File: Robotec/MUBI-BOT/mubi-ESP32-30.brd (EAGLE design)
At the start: 70.2 x 49.5 mm, 35 parts, among them IC1 L293D, IC2 7805T

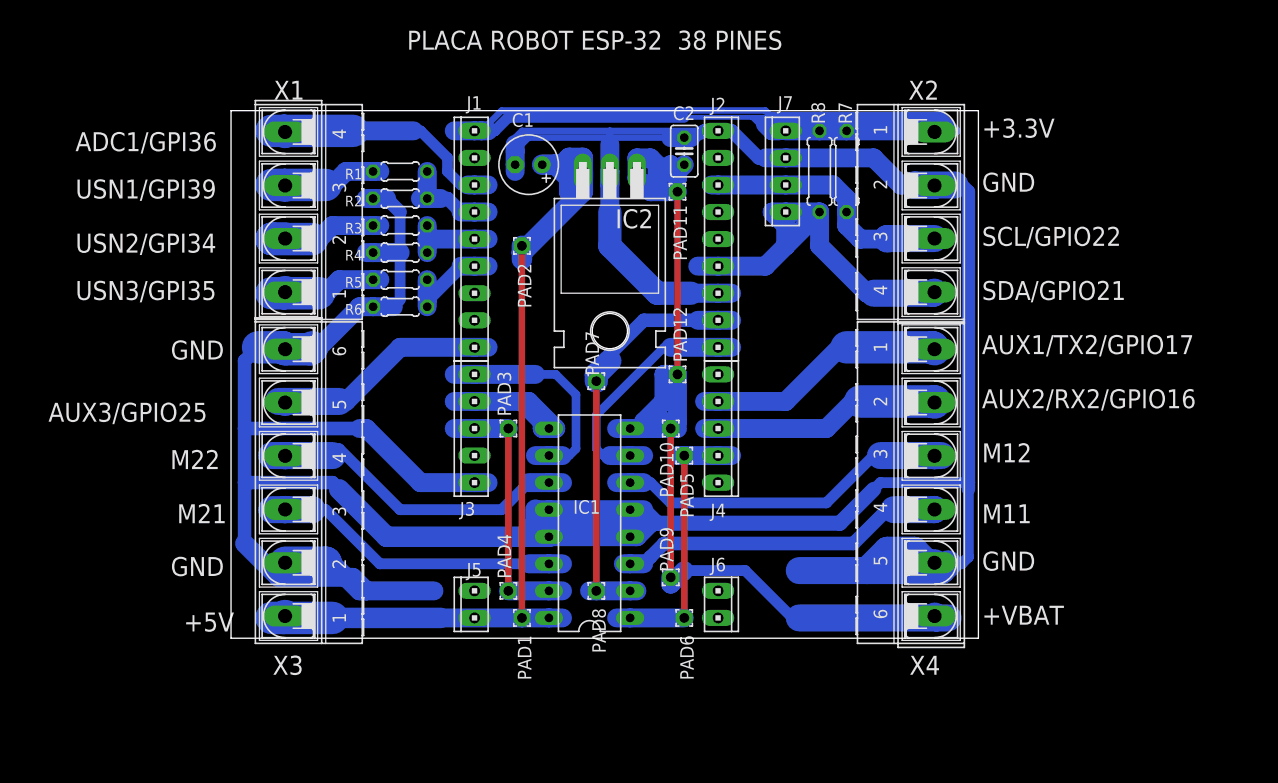
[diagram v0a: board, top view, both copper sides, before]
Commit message: update sch & brd
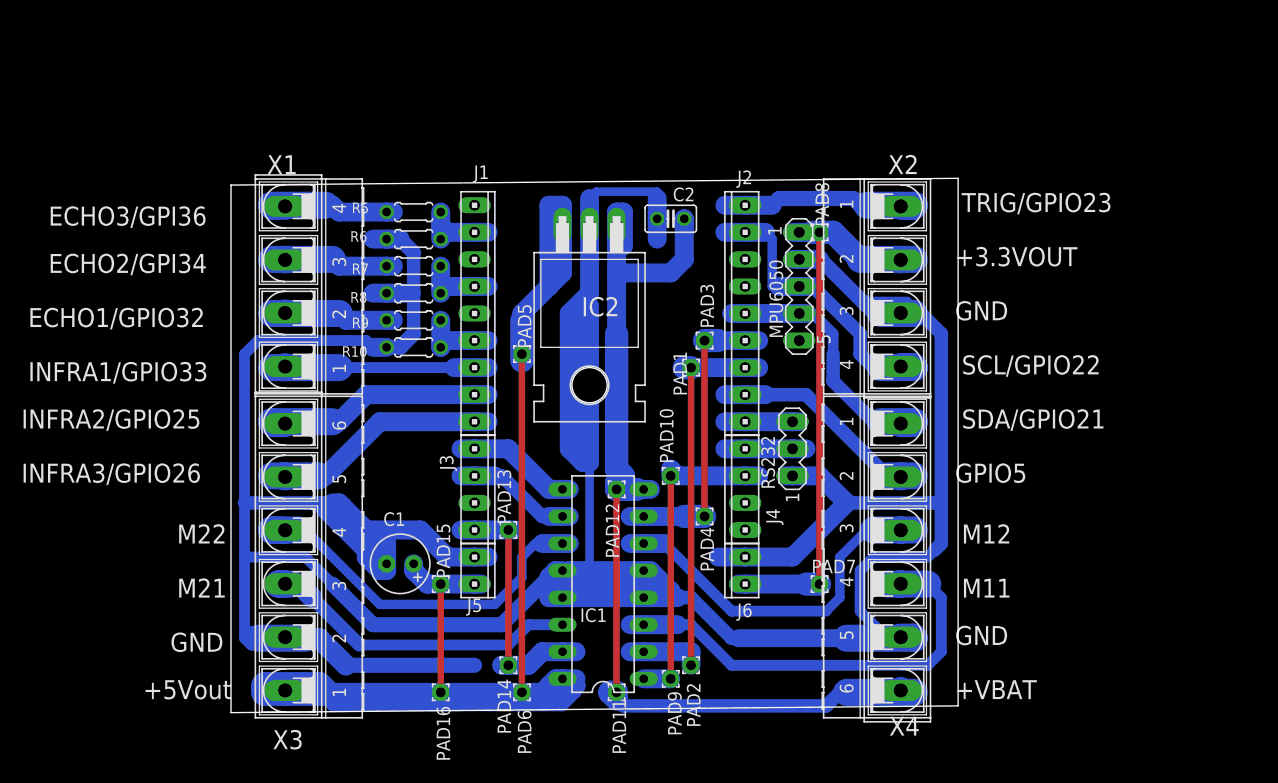
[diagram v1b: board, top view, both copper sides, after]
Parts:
- removed J7: (no value), con-amp:10X04MTA
- removed R1, R3: 5K6, resistor:0204/5
- removed R2, R4: 10K, resistor:0204/5
- added MPU6050: (no value), con-lstb:MA05-1
- added PAD13, PAD14, PAD15, PAD16: WIREPAD1,6/0,9, wirepad:1,6/0,9
- added R10: 10K, resistor:0204/5
- added R9: 5K6, resistor:0204/5
- added RS232: (no value), con-lstb:MA03-1
- C1: value 10uF/16V -> (none)
- C2: value 100nF -> (none)
- J3, J4: device con-amp:10X05MTA -> con-amp:10X04MTA
- R7: value 4K7 -> 5K6; device resistor:0207/7 -> resistor:0204/5
- R8: value 4K7 -> 10K; device resistor:0207/7 -> resistor:0204/5
- moved PAD11 47.3 mm to (36.2, 1.91)
- moved PAD2 42.5 mm to (43.2, 4.45)
- moved R7 41.6 mm to (17.1, 41.9), turned to 0 degrees
- moved R8 39.8 mm to (17.1, 39.4), turned to 180 degrees
- moved PAD8 39.6 mm to (55.2, 45.1)
- moved C1 39.4 mm to (15.9, 14.0)
- moved PAD1 28.4 mm to (43.2, 32.4)
- moved PAD7 28.3 mm to (55.2, 12.1)
- moved PAD3 20.2 mm to (44.5, 34.9)
- moved PAD4 19.7 mm to (44.5, 18.4)
- moved PAD5 18.0 mm to (27.3, 33.7)
- moved PAD6 16.8 mm to (27.3, 1.91)
- moved PAD12 12.2 mm to (36.2, 21.0), turned to 0 degrees
- moved PAD9 9.52 mm to (41.3, 3.17)
- moved X2 7.67 mm to (62.9, 40.0)
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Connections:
- removed net AUX1/TX2: J4.4, X4.1
- removed net AUX2/RX2: J4.3, X4.2
- removed net AUX3: J1.9, X3.5
- removed net N$1: R1.1, X1.3
- removed net N$2: R3.1, X1.2
- removed net N$4: J1.3, X1.4
- removed net USON1: J1.4, R1.2, R2.2
- removed net USON2: J1.5, R3.2, R4.2
- removed net USON3: J1.6, R5.2, R6.2
- new net GPI34: J1.6, R7.2, R8.1
- new net GPI36: J1.8, R5.2, R6.1
- new net GPIO23: J2.1, X2.1
- new net GPIO25: J1.2, X3.6
- new net GPIO26: J1.1, X3.5
- new net GPIO32: J1.4, R10.1, R9.2
- new net GPIO33: J1.3, X1.1
- new net GPIO5: J2.8, X4.2
- new net N$5: R7.1, X1.3
- new net N$8: R9.1, X1.2
- new net RX2: J4.1, RS232.2
- new net TX2: J2.9, RS232.3
- net +3.3V: now also J6.2, MPU6050.1, PAD7.1, PAD8.1, X2.2; no longer J1.1, J7.1, R7.2, R8.2, X2.1
- net +5V: now also J5.1, PAD15.1, PAD16.1, PAD5.1, PAD6.1; no longer J5.2, PAD1.1, PAD2.1
- net +VBAT: no longer PAD10.1, PAD9.1
- net CM11: now also J2.7, PAD1.1, PAD2.1; no longer J2.2, PAD7.1, PAD8.1
- net CM12: now also J2.6, PAD3.1, PAD4.1; no longer J2.1
- net CM21: now also J3.1, PAD13.1, PAD14.1; no longer J3.3, PAD3.1, PAD4.1
- net CM22: now also J3.3; no longer J3.1
- net ENAM1: now also PAD10.1, PAD9.1; no longer PAD5.1, PAD6.1
- net ENAM2: now also J3.4; no longer J3.2
- net GND: now also J5.2, J6.1, MPU6050.2, R10.2, R6.2, R8.2, RS232.1, X2.3; no longer J2.3, J2.9, J3.5, J7.2, R2.1, R4.1, R6.1, X2.2, X3.6
- net N$3: now also X1.4; no longer X1.1
- net SCL: now also J2.2, MPU6050.3, X2.4; no longer J2.7, J7.3, R7.1, X2.3
- net SDA: now also J2.5, MPU6050.4, X4.1; no longer J2.4, J7.4, R8.1, X2.4
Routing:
- net +5V: track 84.6 -> 167.8 mm
- net +3.3V: track 110.5 -> 53.2 mm
- net GND: track 358.7 -> 411.5 mm
- net AUX1/TX2: track 23.8 -> 0.00 mm
- net N$4: track 23.3 -> 0.00 mm
- net AUX2/RX2: track 22.7 -> 0.00 mm
- net GPIO25: track 0.00 -> 22.7 mm
- net GPIO26: track 0.00 -> 22.6 mm
- net AUX3: track 21.9 -> 0.00 mm
- net GPIO5: track 0.00 -> 21.1 mm
- net GPIO33: track 0.00 -> 20.5 mm
- net GPIO23: track 0.00 -> 19.6 mm
- net SDA: track 38.8 -> 25.3 mm
- net N$2: track 12.0 -> 0.00 mm
- net N$5: track 0.00 -> 11.8 mm
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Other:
- board size 70.2 x 49.5 mm -> 68.2 x 50.2 mm
- board text added: "+3.3VOUT"
- board text added: "+5Vout"
- board text added: "ECHO1/GPIO32"
- board text added: "ECHO2/GPI34"
- board text added: "ECHO3/GPI36"
- board text added: "GPIO5"
- board text added: "INFRA1/GPIO33"
- board text added: "INFRA2/GPIO25"
- board text added: "INFRA3/GPIO26"
- board text added: "TRIG/GPIO23"
- board text removed: "+3.3V"
- board text removed: "+5V"
- board text removed: "ADC1/GPI36"
- board text removed: "AUX1/TX2/GPIO17"
- board text removed: "AUX2/RX2/GPIO16"
- board text removed: "AUX3/GPIO25"
- board text removed: "PLACA ROBOT ESP-32 38 PINES"
- board text removed: "USN1/GPI39"
- board text removed: "USN2/GPI34"
- board text removed: "USN3/GPI35"

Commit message: update mubi-bot
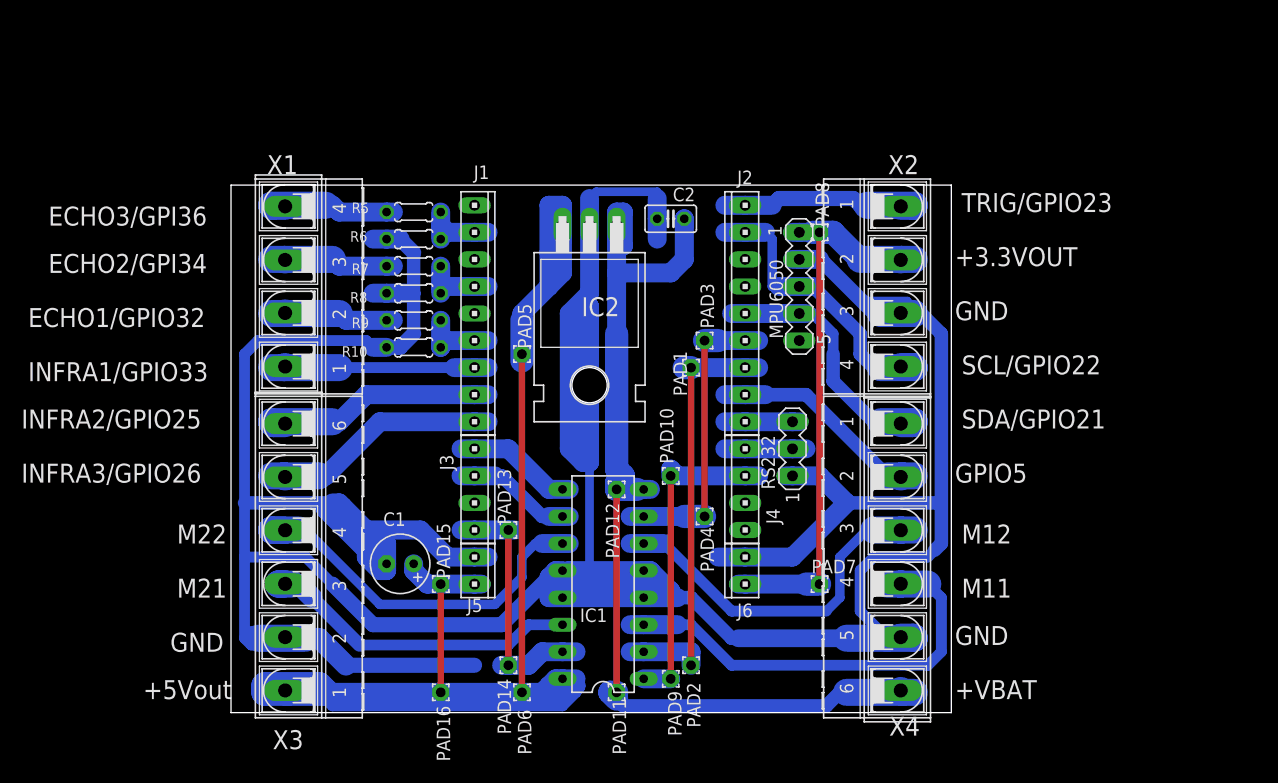
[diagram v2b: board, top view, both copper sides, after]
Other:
- board size 68.2 x 50.2 mm -> 67.6 x 49.5 mm
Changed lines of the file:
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@@
 <board>
 <plain>
-<wire x1="0" y1="0" x2="68.25" y2="0.635" width="0" layer="20"/>
-<wire x1="68.25" y1="0.635" x2="68.25" y2="50.155" width="0" layer="20"/>
-<wire x1="68.25" y1="50.155" x2="0" y2="49.52" width="0" layer="20"/>
+<wire x1="0" y1="0" x2="67.615" y2="0" width="0" layer="20"/>
+<wire x1="67.615" y1="0" x2="67.615" y2="49.52" width="0" layer="20"/>
+<wire x1="67.615" y1="49.52" x2="0" y2="49.52" width="0" layer="20"/>
 <wire x1="0" y1="49.52" x2="0" y2="0" width="0" layer="20"/>
 <dimension x1="0" y1="0" x2="0" y2="49.53" x3="-19.685" y3="24.765" textsize="1.778" layer="1"/>
@@
 <text x="-19.685" y="21.59" size="1.778" layer="25">INFRA3/GPIO26</text>
 <text x="67.945" y="21.59" size="1.778" layer="25">GPIO5</text>
-<dimension x1="22.86" y1="12.065" x2="48.26" y2="12.065" x3="35.56" y3="-3.81" textsize="1.778" layer="1"/>
 </plain>
 <attributes>
